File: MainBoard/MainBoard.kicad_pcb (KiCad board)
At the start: 6 copper layers, 45 x 45.6 mm, 96 parts, among them J1 KH-TYPE-C-16P, Q1 PMV19XNEAR, Q2 PMV19XNEAR, Q3 PMV19XNEAR, Q4 PMV19XNEAR, U1 INA185A4IDRLR, U10 SI3477DV-T1-GE3, U11 INA185A4IDRLR, U12 SI3477DV-T1-GE3, U2 SI3477DV-T1-GE3, U3 STM32L496VGY6PTR, U4 FUSB302BMPX, U5 BNO086, U6 TPS63802DLAR, U7 SI3477DV-T1-GE3, U8 BQ25756ERRVR, U9 TCAN332DCNR, Y1 9HT11-32.768KBZF-T

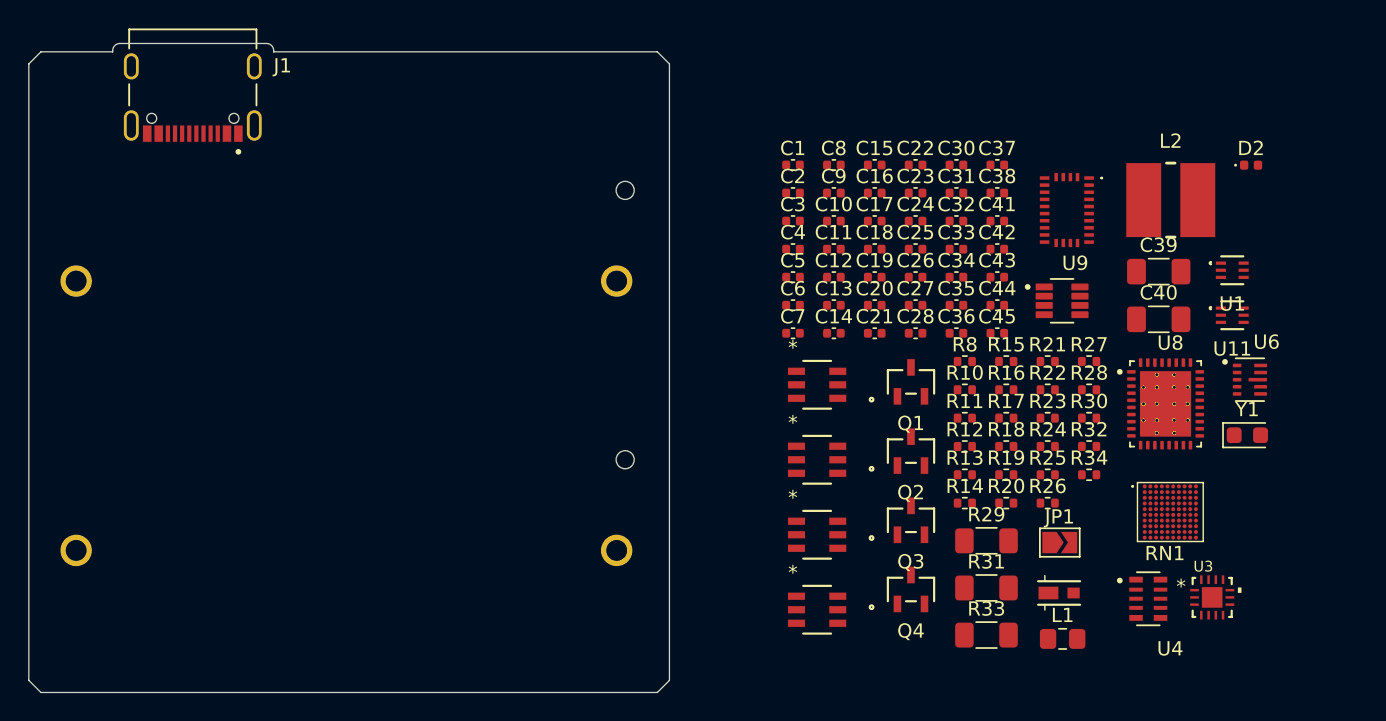
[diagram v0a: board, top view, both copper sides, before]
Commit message: Footprint edits and board setup
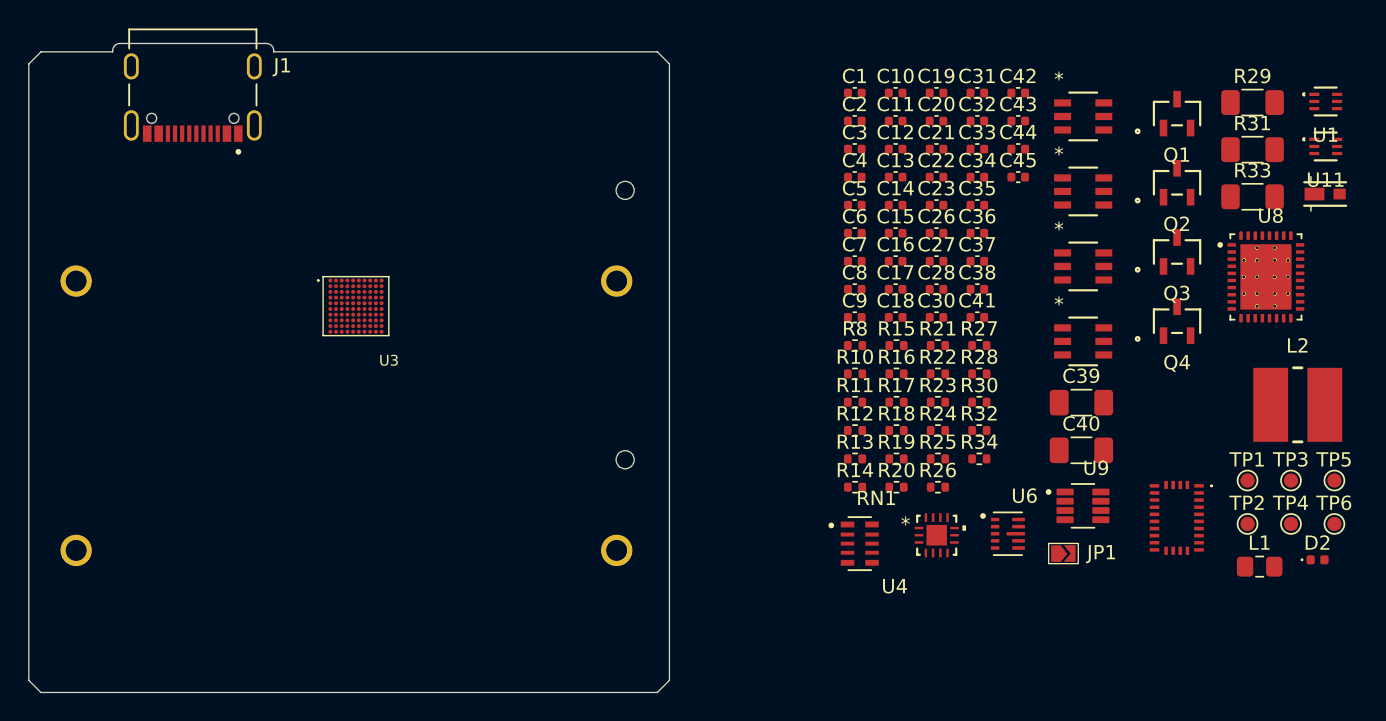
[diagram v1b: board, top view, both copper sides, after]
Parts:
- removed C24, C25: 22pF, Capacitor_SMD:C_0402_1005Metric
- removed Y1: 9HT11-32.768KBZF-T, Crystal:Crystal_SMD_2012-2Pin_2.0x1.2mm_HandSoldering
- added TP1: BatBeforeCutoff, TestPoint:TestPoint_Pad_D1.0mm, F.Cu at (155.0, 71.9)
- added TP2: Bat+, TestPoint:TestPoint_Pad_D1.0mm, F.Cu at (155.0, 74.9)
- added TP3: 3.3V, TestPoint:TestPoint_Pad_D1.0mm, F.Cu at (158.1, 71.9)
- added TP4: GND, TestPoint:TestPoint_Pad_D1.0mm, F.Cu at (158.1, 74.9)
- added TP5: GND, TestPoint:TestPoint_Pad_D1.0mm, F.Cu at (161.1, 71.9)
- added TP6: GND, TestPoint:TestPoint_Pad_D1.0mm, F.Cu at (161.1, 74.9)
- JP1: footprint Jumper:SolderJumper-2_P1.3mm_Open_TrianglePad1.0x1.5mm -> inspirefly:SmallJumper
- R19: value 25k -> 50k
- moved U3 59.0 mm to (92.4, 59.6)
- moved R33 36.0 mm to (155.4, 51.9)
- moved R29 36.0 mm to (155.4, 45.3)
- moved R31 36.0 mm to (155.4, 48.6)
- moved D1 33.7 mm to (160.5, 51.7)
- moved D2 28.1 mm to (159.9, 77.4)
- moved Q1 26.5 mm to (150.1, 46.1)
- moved U10 26.5 mm to (143.5, 56.8)
- moved Q2 26.5 mm to (150.1, 51.0)
- moved Q3 26.5 mm to (150.1, 55.8)
- moved Q4 26.5 mm to (150.1, 60.7)
- moved U2 26.5 mm to (143.5, 46.3)
- moved U7 26.5 mm to (143.5, 51.6)
- moved U12 26.5 mm to (143.5, 62.1)
- moved U5 23.0 mm to (150.0, 74.5)
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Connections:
- C41 pad 2: GND -> Net-(U8-BTST1)
- C42 pad 1: GND -> BAT_SIDE_INDUC
- C42 pad 2: BAT_SIDE_INDUC -> Net-(U8-BTST2)
- U3 pad E1: unconnected-(U3A-PC8-PadE1) -> IMU_MCO
- U5 pad 10: unconnected-(U5-CLKSEL0-Pad10) -> +3.3V
- U5 pad 17: unconnected-(U5-SA0/H_MOSI-Pad17) -> H_MDSI_MCUMOSI
- U5 pad 18: unconnected-(U5-H_CSN-Pad18) -> IMU_CSN_GPIO
- U5 pad 19: unconnected-(U5-H_SCL/SCK/RX-Pad19) -> IMU_MCU_SLK
- U5 pad 20: unconnected-(U5-H_SDA/H_MISO/TX-Pad20) -> IMU_MCU_MISO
- U5 pad 26: Net-(U5-XOUT32/CLKSEL1) -> +3.3V
- U5 pad 27: Net-(U5-XIN32) -> IMU_MCO
- U8 pad 20: BAT_SIDE_INDUC -> Net-(U8-BTST2)
- U8 pad 26: EXTERNAL_SIDE_INDUC -> Net-(U8-BTST1)
